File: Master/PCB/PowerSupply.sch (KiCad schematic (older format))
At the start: 35 parts, among them J13 Charger 12V, Q2 BSS138, Q28 BSS138, Q29 BSS138, Q30 BSS138, U19 LM5165YDRC

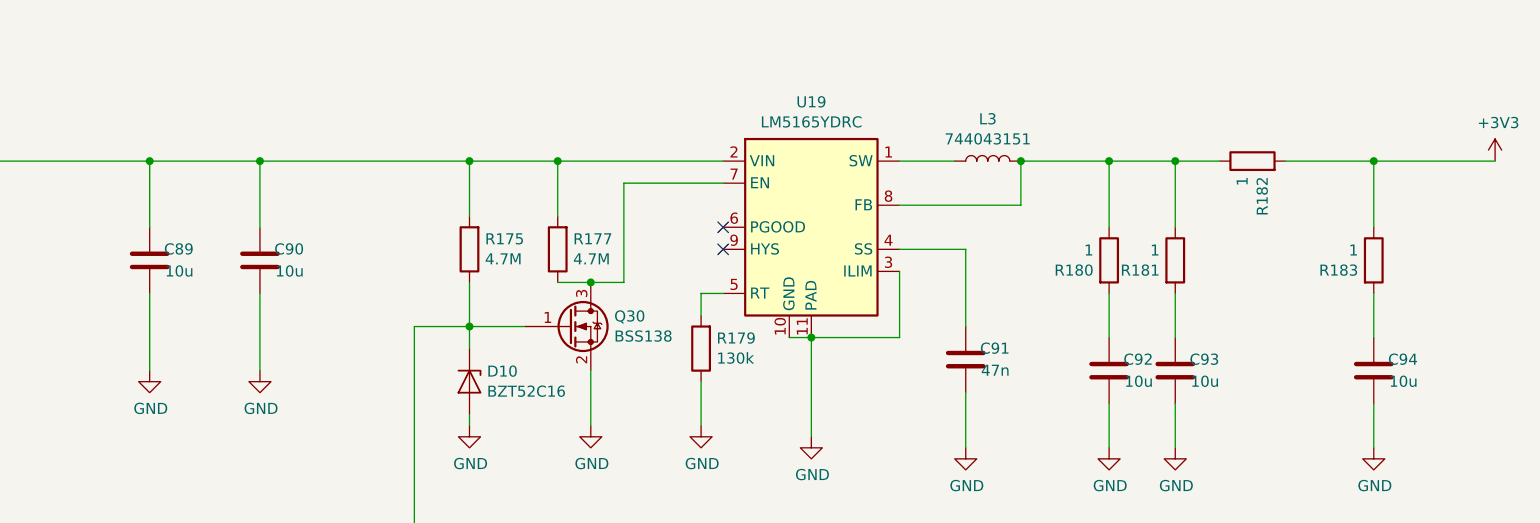
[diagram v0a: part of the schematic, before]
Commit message: Datasheet update for V1.0
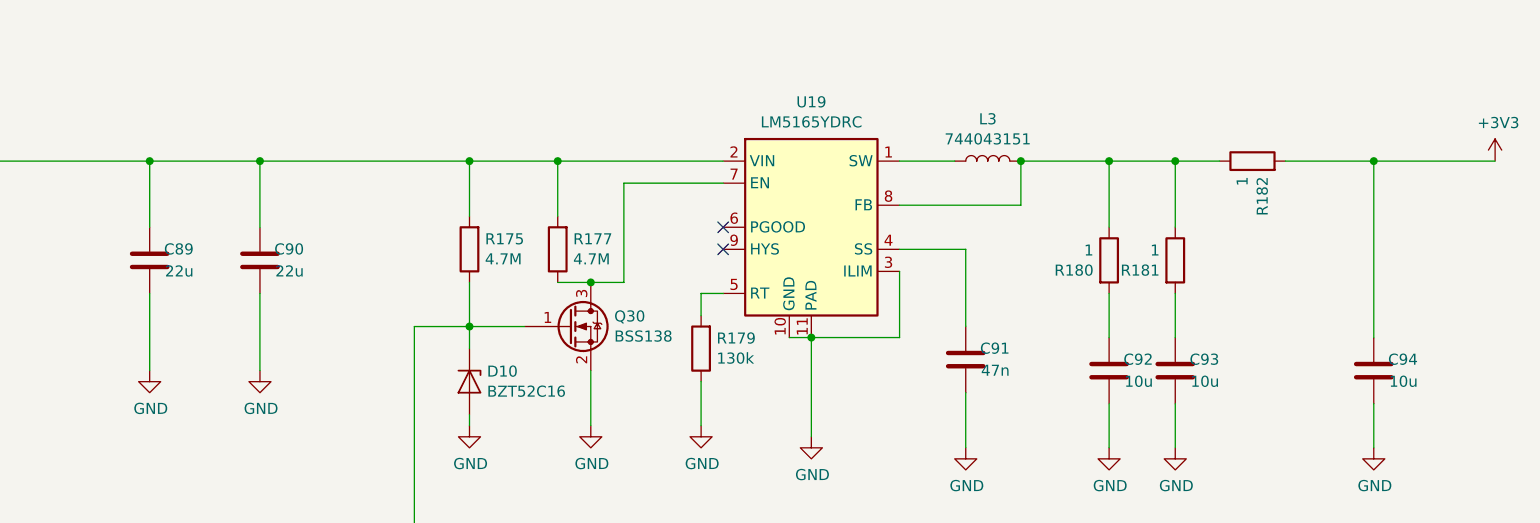
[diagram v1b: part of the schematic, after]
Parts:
- removed R183: 1, Resistors_SMD:R_0603_HandSoldering, symbol BMS-Master-rescue:R-Device-BMS-Master-rescue
- C88: MPN (none) -> GRM188R61A225KE34D
- C89, C90: value 10u -> 22u; MPN (none) -> CL21A226MOQNNNE; Volatge 50V -> (none)
- C91: MPN (none) -> GCM188R71H473KA55D; Volatge 50V -> (none); Voltage (none) -> 100V
- C92, C93, C94: MPN (none) -> CL10A106MQ8NNNC; Volatge 50V -> (none)
- D10, D7: MPN (none) -> BZT52C16-E3-08
- D11, D12, D13, D8, D9: MPN (none) -> 1N4148W-7-F
- D6: MPN (none) -> N/A
- J13: MPN (none) -> 282834-2
- L3: MPN (none) -> 744043151
- Q2, Q28, Q29, Q30: MPN (none) -> BSS138
- R172: MPN (none) -> RC0603FR-07100RL
- R173, R176, R178, R41: MPN (none) -> RC0603FR-0710KL
- R174: MPN (none) -> RC0603JR-071ML
- R175, R177: MPN (none) -> RC0603FR-074M7L
- R179: MPN (none) -> RC0603FR-07130KL
- R180, R181, R182: MPN (none) -> RC0603FR-071RL
- U19: MPN (none) -> LM5165YDRCT
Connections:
- net +3V3: now also C94.2
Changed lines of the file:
@@
 F 2 "Housings_SON:Texas_S-PVSON-N10_ThermalVias" H 14950 6250 50  0001 L CNN
 F 3 "http://www.ti.com/lit/ds/symlink/lm5165.pdf" H 14900 7250 50  0001 C CNN
+F 4 "LM5165YDRCT" H 14900 6700 50  0001 C CNN "MPN"
 	1    14900 6700
 	1    0    0    -1
@@
 P 12400 6850
 F 0 "C90" H 12200 6800 50  0000 L CNN
-F 1 "10u" H 12200 6900 50  0000 L CNN
+F 1 "22u" H 12200 6900 50  0000 L CNN
 F 2 "Capacitors_SMD:C_0805_HandSoldering" H 12438 6700 50  0001 C CNN
 F 3 "~" H 12400 6850 50  0001 C CNN
-F 4 "50V" H 12400 6850 50  0001 C CNN "Volatge"
+F 4 "CL21A226MOQNNNE" H 12400 6850 50  0001 C CNN "MPN"
 	1    12400 6850
 	-1   0    0    1
@@
 P 11900 6850
 F 0 "C89" H 11700 6800 50  0000 L CNN
-F 1 "10u" H 11700 6900 50  0000 L CNN
+F 1 "22u" H 11700 6900 50  0000 L CNN
 F 2 "Capacitors_SMD:C_0805_HandSoldering" H 11938 6700 50  0001 C CNN
 F 3 "~" H 11900 6850 50  0001 C CNN
-F 4 "50V" H 11900 6850 50  0001 C CNN "Volatge"
+F 4 "CL21A226MOQNNNE" H 11900 6850 50  0001 C CNN "MPN"
 	1    11900 6850
 	-1   0    0    1
@@
 F 2 "TO_SOT_Packages_SMD:SOT-23" H 14000 7075 50  0001 L CIN
 F 3 "https://www.fairchildsemi.com/datasheets/BS/BSS138.pdf" H 13800 7150 50  0001 L CNN
+F 4 "BSS138" H 13800 7150 50  0001 C CNN "MPN"
 	1    13800 7150
 	1    0    0    -1
@@
 F 2 "Resistors_SMD:R_0603_HandSoldering" V 14330 7250 50  0001 C CNN
 F 3 "~" H 14400 7250 50  0001 C CNN
+F 4 "RC0603FR-07130KL" H 14400 7250 50  0001 C CNN "MPN"
 	1    14400 7250
 	-1   0    0    1
@@
 F 2 "Resistors_SMD:R_0603_HandSoldering" V 13680 6800 50  0001 C CNN
 F 3 "~" H 13750 6800 50  0001 C CNN
+F 4 "RC0603FR-074M7L" H 13750 6800 50  0001 C CNN "MPN"
 	1    13750 6800
 	-1   0    0    1
@@
 F 2 "Resistors_SMD:R_0603_HandSoldering" V 13280 6800 50  0001 C CNN
 F 3 "~" H 13350 6800 50  0001 C CNN
+F 4 "RC0603FR-074M7L" H 13350 6800 50  0001 C CNN "MPN"
 	1    13350 6800
 	-1   0    0    1
@@
 F 2 "Inductors_SMD:L_Wuerth_WE-PD2-Typ-MS" H 15700 6400 50  0001 C CNN
 F 3 "~" H 15700 6400 50  0001 C CNN
+F 4 "744043151" H 15700 6400 50  0001 C CNN "MPN"
 	1    15700 6400
 	0    -1   -1   0
@@
 F 2 "Resistors_SMD:R_0603_HandSoldering" V 13580 10850 50  0001 C CNN
 F 3 "~" H 13650 10850 50  0001 C CNN
+F 4 "RC0603FR-0710KL" H 13650 10850 50  0001 C CNN "MPN"
 	1    13650 10850
 	1    0    0    -1
@@
 F 2 "Resistors_SMD:R_0603_HandSoldering" V 16830 6400 50  0001 C CNN
 F 3 "~" H 16900 6400 50  0001 C CNN
+F 4 "RC0603FR-071RL" H 16900 6400 50  0001 C CNN "MPN"
 	1    16900 6400
 	0    -1   -1   0
@@
 F 2 "Resistors_SMD:R_0603_HandSoldering" V 16180 6850 50  0001 C CNN
 F 3 "~" H 16250 6850 50  0001 C CNN
+F 4 "RC0603FR-071RL" H 16250 6850 50  0001 C CNN "MPN"
 	1    16250 6850
 	1    0    0    -1
@@
 F 2 "Capacitors_SMD:C_0603_HandSoldering" H 16288 7200 50  0001 C CNN
 F 3 "~" H 16250 7350 50  0001 C CNN
-F 4 "50V" H 16250 7350 50  0001 C CNN "Volatge"
+F 4 "" H 16250 7350 50  0001 C CNN "Volatge"
+F 5 "CL10A106MQ8NNNC" H 16250 7350 50  0001 C CNN "MPN"
 	1    16250 7350
 	-1   0    0    1
@@
 F 2 "Capacitors_SMD:C_0603_HandSoldering" H 16588 7200 50  0001 C CNN
 F 3 "~" H 16550 7350 50  0001 C CNN
-F 4 "50V" H 16550 7350 50  0001 C CNN "Volatge"
+F 4 "" H 16550 7350 50  0001 C CNN "Volatge"
+F 5 "CL10A106MQ8NNNC" H 16550 7350 50  0001 C CNN "MPN"
 	1    16550 7350
 	-1   0    0    1
@@
 F 2 "Resistors_SMD:R_0603_HandSoldering" V 16480 6850 50  0001 C CNN
 F 3 "~" H 16550 6850 50  0001 C CNN
+F 4 "RC0603FR-071RL" H 16550 6850 50  0001 C CNN "MPN"
 	1    16550 6850
 	1    0    0    -1
 $EndComp
-Wire Wire Line
-	17450 7000 17450 7200
 Wire Wire Line
 	17450 7500 17450 7700
@@
 F 2 "Capacitors_SMD:C_0603_HandSoldering" H 17488 7200 50  0001 C CNN
 F 3 "~" H 17450 7350 50  0001 C CNN
-F 4 "50V" H 17450 7350 50  0001 C CNN "Volatge"
+F 4 "" H 17450 7350 50  0001 C CNN "Volatge"
+F 5 "CL10A106MQ8NNNC" H 17450 7350 50  0001 C CNN "MPN"
 	1    17450 7350
 	-1   0    0    1
@@
 	1    0    0    -1
 $EndComp
-$Comp
-L BMS-Master-rescue:R-Device-BMS-Master-rescue R183
-U 1 1 5C773AD4
-P 17450 6850
-F 0 "R183" H 17380 6804 50  0000 R CNN
-F 1 "1" H 17380 6895 50  0000 R CNN
-F 2 "Resistors_SMD:R_0603_HandSoldering" V 17380 6850 50  0001 C CNN
-F 3 "~" H 17450 6850 50  0001 C CNN
-	1    17450 6850
-	1    0    0    -1
-$EndComp
 Wire Wire Line
 	17050 6400 17450 6400
-Wire Wire Line
-	17450 6400 17450 6700
 Wire Wire Line
 	15300 6900 15300 7200
@@
 F 2 "Capacitors_SMD:C_0603_HandSoldering" H 15638 7150 50  0001 C CNN
 F 3 "~" H 15600 7300 50  0001 C CNN
-F 4 "50V" H 15600 7300 50  0001 C CNN "Volatge"
+F 4 "100V" H 15600 7300 50  0001 C CNN "Voltage"
+F 5 "GCM188R71H473KA55D" H 15600 7300 50  0001 C CNN "MPN"
 	1    15600 7300
 	-1   0    0    1
@@
 	1    0    0    -1
 $EndComp
-Wire Wire Line
-	17450 6400 18000 6400
 Connection ~ 17450 6400
 $Comp
@@
 F 2 "Resistors_SMD:R_0603_HandSoldering" V 11480 10150 50  0001 C CNN
 F 3 "~" H 11550 10150 50  0001 C CNN
+F 4 "RC0603JR-071ML" H 11550 10150 50  0001 C CNN "MPN"
 	1    11550 10150
 	0    -1   -1   0
@@
 F 3 "~" H 11550 9800 50  0001 C CNN
 F 4 "50V" H 11550 9800 50  0001 C CNN "Volatge"
+F 5 "GRM188R61A225KE34D" H 11550 9800 50  0001 C CNN "MPN"
 	1    11550 9800
 	0    -1   -1   0
@@
 F 2 "TO_SOT_Packages_SMD:SOT-23" H 9950 10325 50  0001 L CIN
 F 3 "https://www.fairchildsemi.com/datasheets/BS/BSS138.pdf" H 9750 10400 50  0001 L CNN
+F 4 "BSS138" H 9750 10400 50  0001 C CNN "MPN"
 	1    9750 10400
 	-1   0    0    -1
@@
 F 2 "Resistors_SMD:R_0603_HandSoldering" V 9830 9800 50  0001 C CNN
 F 3 "~" H 9900 9800 50  0001 C CNN
+F 4 "RC0603FR-07100RL" H 9900 9800 50  0001 C CNN "MPN"
 	1    9900 9800
 	0    -1   -1   0
@@
 F 2 "Resistors_SMD:R_0603_HandSoldering" V 10730 9150 50  0001 C CNN
 F 3 "~" H 10800 9150 50  0001 C CNN
+F 4 "RC0603FR-0710KL" H 10800 9150 50  0001 C CNN "MPN"
 	1    10800 9150
 	0    -1   -1   0
@@
 F 2 "Diodes_SMD:D_SOD-123" H 13550 8325 50  0001 C CNN
 F 3 "https://www.vishay.com/docs/85748/1n4148w.pdf" H 13550 8500 50  0001 C CNN
+F 4 "1N4148W-7-F" H 13550 8500 50  0001 C CNN "MPN"
 	1    13550 8500
 	-1   0    0    1
@@
 F 2 "Diodes_SMD:D_SOD-123" H 13600 8925 50  0001 C CNN
 F 3 "https://www.vishay.com/docs/85748/1n4148w.pdf" H 13600 9100 50  0001 C CNN
+F 4 "1N4148W-7-F" H 13600 9100 50  0001 C CNN "MPN"
 	1    13600 9100
 	-1   0    0    1
@@
 F 2 "Diodes_SMD:D_SOD-123" H 13600 9625 50  0001 C CNN
 F 3 "https://www.vishay.com/docs/85748/1n4148w.pdf" H 13600 9800 50  0001 C CNN
+F 4 "1N4148W-7-F" H 13600 9800 50  0001 C CNN "MPN"
 	1    13600 9800
 	-1   0    0    1
@@
 F 2 "Diodes_SMD:D_SOD-123" H 12450 9625 50  0001 C CNN
 F 3 "https://www.vishay.com/docs/85748/1n4148w.pdf" H 12450 9800 50  0001 C CNN
+F 4 "1N4148W-7-F" H 12450 9800 50  0001 C CNN "MPN"
 	1    12450 9800
 	1    0    0    -1
@@
 F 2 "Diodes_SMD:D_SOD-123" H 11250 8975 50  0001 C CNN
 F 3 "https://www.vishay.com/docs/85748/1n4148w.pdf" H 11250 9150 50  0001 C CNN
+F 4 "1N4148W-7-F" H 11250 9150 50  0001 C CNN "MPN"
 	1    11250 9150
 	1    0    0    -1
@@
 F 2 "Diodes_SMD:D_SOD-123" H 10900 10375 50  0001 C CNN
 F 3 "https://diotec.com/tl_files/diotec/files/pdf/datasheets/bzt52b2v4.pdf" H 10900 10550 50  0001 C CNN
+F 4 "BZT52C16-E3-08" H 10900 10550 50  0001 C CNN "MPN"
 	1    10900 10550
 	0    1    1    0
@@
 F 2 "Diodes_SMD:D_SOD-123" H 13350 7225 50  0001 C CNN
 F 3 "https://diotec.com/tl_files/diotec/files/pdf/datasheets/bzt52b2v4.pdf" H 13350 7400 50  0001 C CNN
+F 4 "BZT52C16-E3-08" H 13350 7400 50  0001 C CNN "MPN"
 	1    13350 7400
 	0    1    1    0
@@
 F 2 "TO_SOT_Packages_SMD:SOT-23" H 13400 10625 50  0001 L CIN
 F 3 "https://www.fairchildsemi.com/datasheets/BS/BSS138.pdf" H 13200 10700 50  0001 L CNN
+F 4 "BSS138" H 13200 10700 50  0001 C CNN "MPN"
 	1    13200 10700
 	-1   0    0    -1
@@
 F 2 "Connectors_Molex:Molex_KK-6410-02_02x2.54mm_Straight" H 8650 7550 50  0001 C CNN
 F 3 "~" H 8650 7550 50  0001 C CNN
+F 4 "282834-2 " H 8650 7550 50  0001 C CNN "MPN"
 	1    8650 7550
 	-1   0    0    -1
@@
 	10250 7550 10250 6400
 Connection ~ 10250 6400
-Wire Wire Line
-	10250 6400 11900 6400
 $Comp
 L BMS-Master-rescue:R-Device-BMS-Master-rescue R178
@@
 F 2 "Resistors_SMD:R_0603_HandSoldering" V 14080 9100 50  0001 C CNN
 F 3 "~" H 14150 9100 50  0001 C CNN
+F 4 "RC0603FR-0710KL" H 14150 9100 50  0001 C CNN "MPN"
 	1    14150 9100
 	0    -1   -1   0
@@
 F 2 "Diode_SMD:D_SMB" H 9700 7375 50  0001 C CNN
 F 3 "http://www.jameco.com/Jameco/Products/ProdDS/1538777.pdf" H 9700 7550 50  0001 C CNN
+F 4 "N/A" H 9700 7550 50  0001 C CNN "MPN"
 	1    9700 7550
 	-1   0    0    1
@@
 F 2 "TO_SOT_Packages_SMD:SOT-23" H 9800 8125 50  0001 L CIN
 F 3 "https://www.fairchildsemi.com/datasheets/BS/BSS138.pdf" H 9600 8200 50  0001 L CNN
+F 4 "BSS138" H 9600 8200 50  0001 C CNN "MPN"
 	1    9600 8200
 	1    0    0    -1
@@
 F 2 "Resistors_SMD:R_0603_HandSoldering" V 9180 8350 50  0001 C CNN
 F 3 "~" H 9250 8350 50  0001 C CNN
+F 4 "RC0603FR-0710KL" H 9250 8350 50  0001 C CNN "MPN"
 	1    9250 8350
 	1    0    0    -1
@@
 Wire Wire Line
 	9700 8000 10050 8000
+Wire Wire Line
+	17450 6400 17450 7200
+Wire Wire Line
+	10250 6400 11900 6400
+Wire Wire Line
+	17450 6400 18000 6400
 $EndSCHEMATC
